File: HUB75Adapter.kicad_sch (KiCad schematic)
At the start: 16 parts, among them J1 Panel 1, J2 Panel 2, J3 P0_SELECT_PIN4, J4 P0_SELECT_PIN8, J5 P1_SELECT_PIN4, J6 P1_SELECT_PIN8, U1 RaspberryPi Zero W, U2 74HCT245, U3 74HCT245, U4 74HCT245

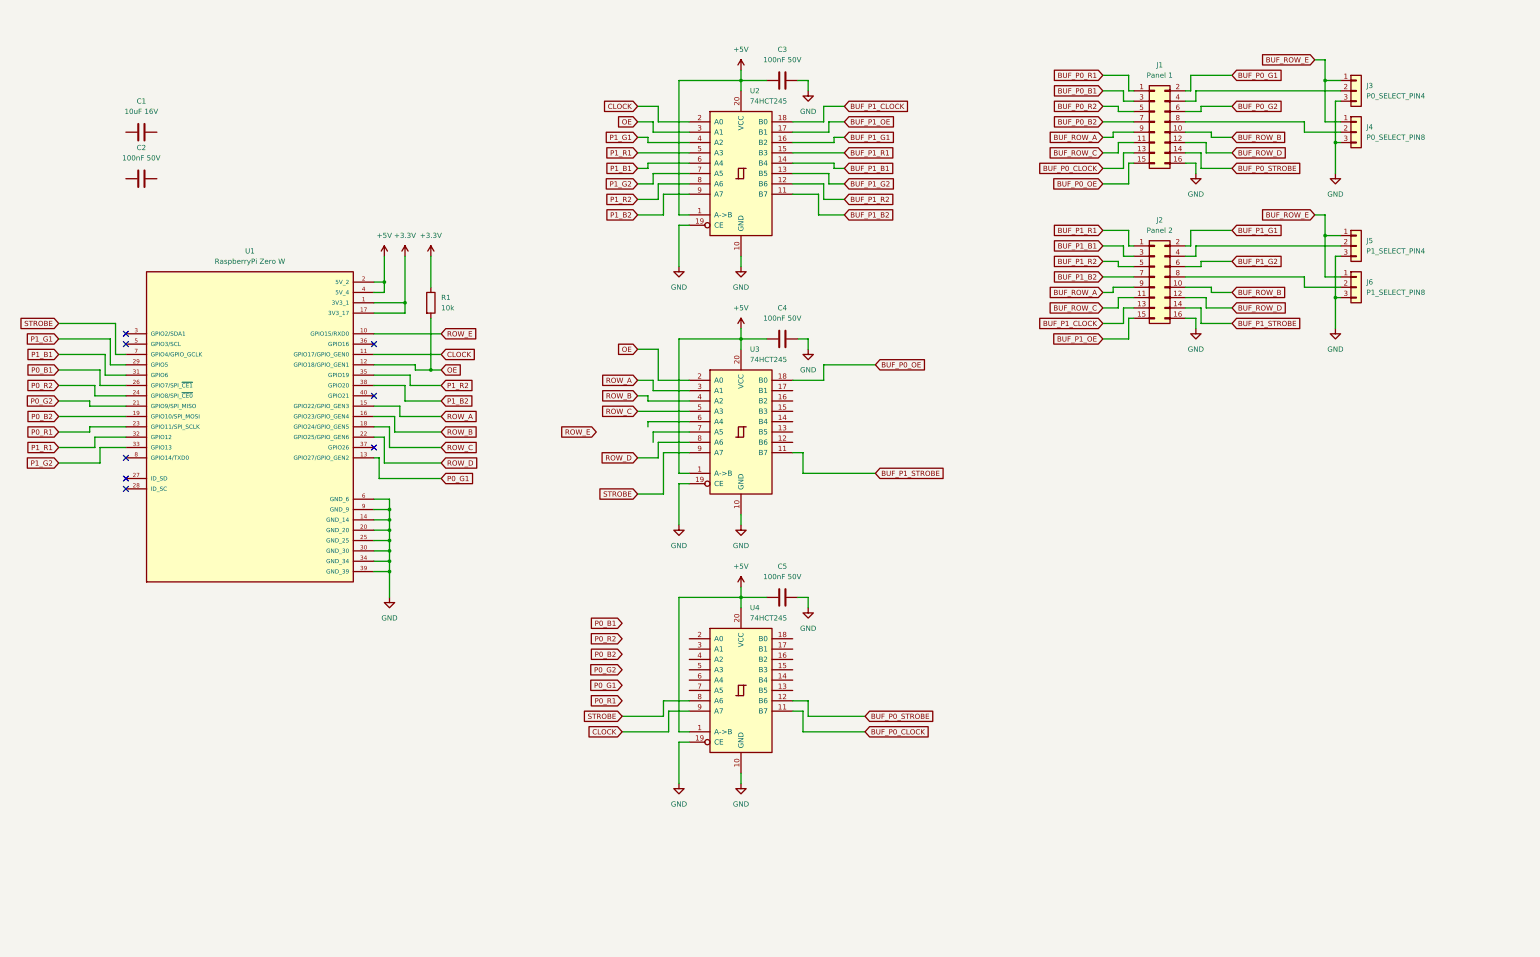
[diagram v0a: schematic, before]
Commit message: Add README. Board updates.
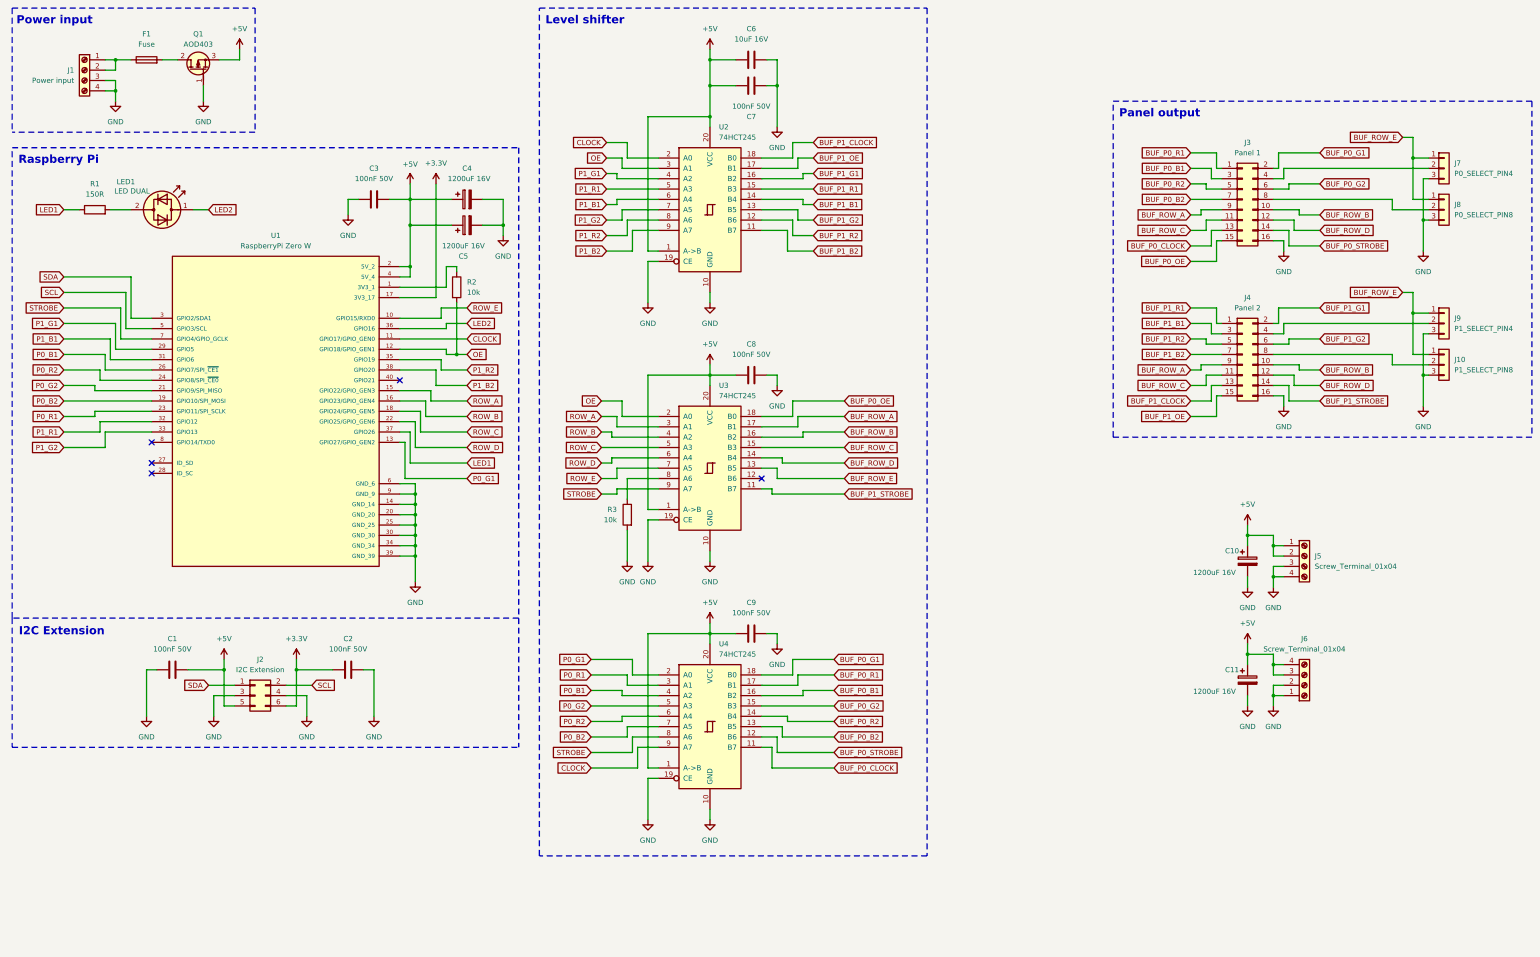
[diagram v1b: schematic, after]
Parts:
- added C1, C2: 100nF 50V, Capacitor_SMD:C_1206_3216Metric_Pad1.33x1.80mm_HandSolder, symbol Device:C
- added C10, C11, C4, C5: 1200uF 16V, Capacitor_THT:CP_Radial_D10.0mm_P5.00mm, symbol Device:C_Polarized
- added F1: Fuse, Fuse:Fuseholder_Littelfuse_Nano2_154x, symbol Device:Fuse
- added J1: Power input, TerminalBlock_Phoenix:TerminalBlock_Phoenix_MKDS-1,5-4_1x04_P5.00mm_Horizontal, symbol Connector:Screw_Terminal_01x04
- added J2: I2C Extension, Connector_IDC:IDC-Header_2x03_P2.54mm_Vertical, symbol Connector_Generic:Conn_02x03_Odd_Even
- added J5, J6: Screw_Terminal_01x04, TerminalBlock_Phoenix:TerminalBlock_Phoenix_MKDS-1,5-4_1x04_P5.00mm_Horizontal, symbol Connector:Screw_Terminal_01x04
- added LED1: LED DUAL, PCM_LED_THT_AKL:LED_D3.0mm_BiDir, symbol Device:LED_Dual_Bidirectional
- added Q1: AOD403, PCM_Package_TO_SOT_SMD_AKL:TO-252-2, symbol PCM_Transistor_MOSFET_AKL:AOD403
- added R1: 150R, PCM_Resistor_SMD_AKL:R_1206_3216Metric_Pad1.42x1.75mm_HandSolder, symbol Device:R
- added R3: 10k, PCM_Resistor_SMD_AKL:R_1206_3216Metric_Pad1.42x1.75mm_HandSolder, symbol Device:R
- renumbered C2 to C3, C1 to C6, C3 to C7, C4 to C8, C5 to C9, J6 to J10, J1 to J3, J2 to J4, J3 to J7, J4 to J8, J5 to J9, R1 to R2
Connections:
- net +3.3V: now also C2.2, J2.6 (Pin_6); no longer R2.1, U1.1 (3V3_1)
- net +5V: now also C3.2, C6.1, C1.1, C10.1, C11.1, C4.1, C5.1, J2.5 (Pin_5), J5.1 (Pin_1), J5.2 (Pin_2), J6.3 (Pin_3), J6.4 (Pin_4), Q1.3 (S)
- net BUF_P0_B1: now also U4.16 (B2)
- net BUF_P0_B2: now also U4.13 (B5)
- net BUF_P0_G1: now also U4.18 (B0)
- net BUF_P0_G2: now also U4.15 (B3)
- net BUF_P0_R1: now also U4.17 (B1)
- net BUF_P0_R2: now also U4.14 (B4)
- net BUF_ROW_A: now also U3.17 (B1)
- net BUF_ROW_B: now also U3.16 (B2)
- net BUF_ROW_C: now also U3.15 (B3)
- net BUF_ROW_D: now also U3.14 (B4)
- net BUF_ROW_E: now also U3.13 (B5)
- net GND: now also C3.1, C6.2, C1.2, C10.2, C11.2, C2.1, C4.2, C5.2, J1.3 (Pin_3), J1.4 (Pin_4), J2.3 (Pin_3), J2.4 (Pin_4), J5.3 (Pin_3), J5.4 (Pin_4), J6.1 (Pin_1), J6.2 (Pin_2), Q1.1 (G), R3.2
- net P0_B1: now also U4.4 (A2)
- net P0_B2: now also U4.7 (A5)
- net P0_G1: now also U4.2 (A0)
- net P0_G2: now also U4.5 (A3)
- net P0_R1: now also U4.3 (A1)
- net P0_R2: now also U4.6 (A4)
- net ROW_D: now also U3.6 (A4); no longer U3.8 (A6)
- net ROW_E: now also U3.7 (A5)
- net SDA: now reaches U1.3 (GPIO2/SDA1)
- net SDA: now also J2.1 (Pin_1)
- net LED2: now reaches U1.36 (GPIO16)
- net LED2: now also LED1.1 (KA)
- net LED1: now reaches U1.37 (GPIO26)
- net LED1: now also R1.1
- net SCL: now reaches U1.5 (GPIO3/SCL)
- net SCL: now also J2.2 (Pin_2)
- new net: F1.1, J1.1 (Pin_1), J1.2 (Pin_2)
- new net: F1.2, Q1.2 (D)
- new net: R2.1, U1.1 (3V3_1)
- new net: LED1.2 (AK), R1.2
- new net: R3.1, U3.8 (A6)
- no-connect marks 8 -> 5
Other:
- note added: "I2C Extension"
- note added: "Level shifter"
- note added: "Panel output"
- note added: "Power input"
- note added: "Raspberry Pi"
- title: HUB75 LED-Matrix Adapter -> HUB75(E) LED-Matrix Adapter
- moved on the sheet: C3, C6, C7, C8, C9, J10, J3, J4, J7, J8, J9, R2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

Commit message: Finish board
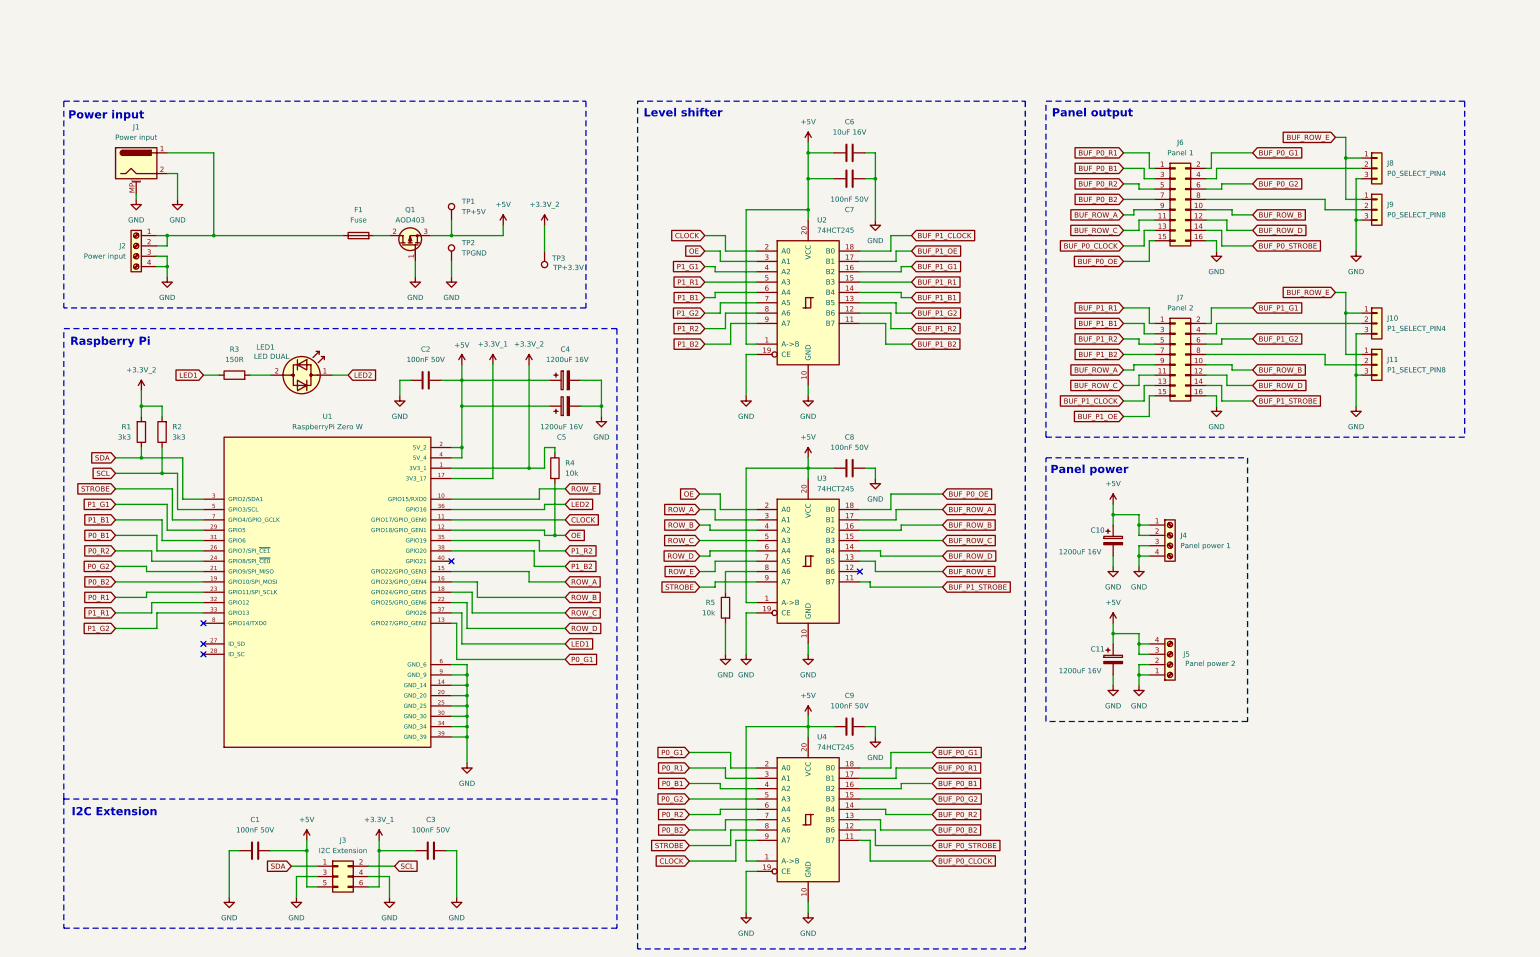
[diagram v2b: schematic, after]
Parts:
- added J1: Power input, Connector_BarrelJack:BarrelJack_Horizontal, symbol Connector:Barrel_Jack_MountingPin
- added R1, R2: 3k3, PCM_Resistor_SMD_AKL:R_1206_3216Metric_Pad1.42x1.75mm_HandSolder, symbol Device:R
- added TP1: TP+5V, TestPoint:TestPoint_Pad_D1.0mm, symbol Connector:TestPoint
- added TP2: TPGND, TestPoint:TestPoint_Pad_D1.0mm, symbol Connector:TestPoint
- added TP3: TP+3.3V, TestPoint:TestPoint_Pad_D1.0mm, symbol Connector:TestPoint
- C1, C6, C7, C8, C9: footprint Capacitor_SMD:C_1206_3216Metric_Pad1.33x1.80mm_HandSolder -> PCM_Capacitor_SMD_AKL:C_1206_3216Metric_Pad1.42x1.75mm_HandSolder
- C2: renamed from C3; footprint Capacitor_SMD:C_1206_3216Metric_Pad1.33x1.80mm_HandSolder -> PCM_Capacitor_SMD_AKL:C_1206_3216Metric_Pad1.42x1.75mm_HandSolder
- C3: renamed from C2; footprint Capacitor_SMD:C_1206_3216Metric_Pad1.33x1.80mm_HandSolder -> PCM_Capacitor_SMD_AKL:C_1206_3216Metric_Pad1.42x1.75mm_HandSolder
- J4: renamed from J5; value Screw_Terminal_01x04 -> Panel power 1
- J5: renamed from J6; value Screw_Terminal_01x04 -> Panel power 2
- renumbered J9 to J10, J10 to J11, J1 to J2, J2 to J3, J3 to J6, J4 to J7, J7 to J8, J8 to J9, R1 to R3, R2 to R4, R3 to R5
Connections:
- net +5V: now also TP1.1
- net GND: now also J1.2, J1.MP (MountPin), TP2.1
- net SCL: now also R2.1
- net SDA: now also R1.1
- net at F1.1, J2.1 (Pin_1), J2.2 (Pin_2): now also J1.1
- net +3.3V_2: now reaches R4.1, U1.1 (3V3_1)
- net +3.3V_2: now also R1.2, R2.2, TP3.1
- net +3.3V renamed +3.3V_1
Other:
- note added: "Panel power"
- moved on the sheet: C1, C10, C11, C2, C3, C4, C5, C6, C7, C8, C9, F1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
